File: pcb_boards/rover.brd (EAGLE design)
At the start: 2.5 x 2.5 mm, 16 parts, among them IC1 MC33269ST-5.0T3, J1 B02B-PASK(LF)(SN)

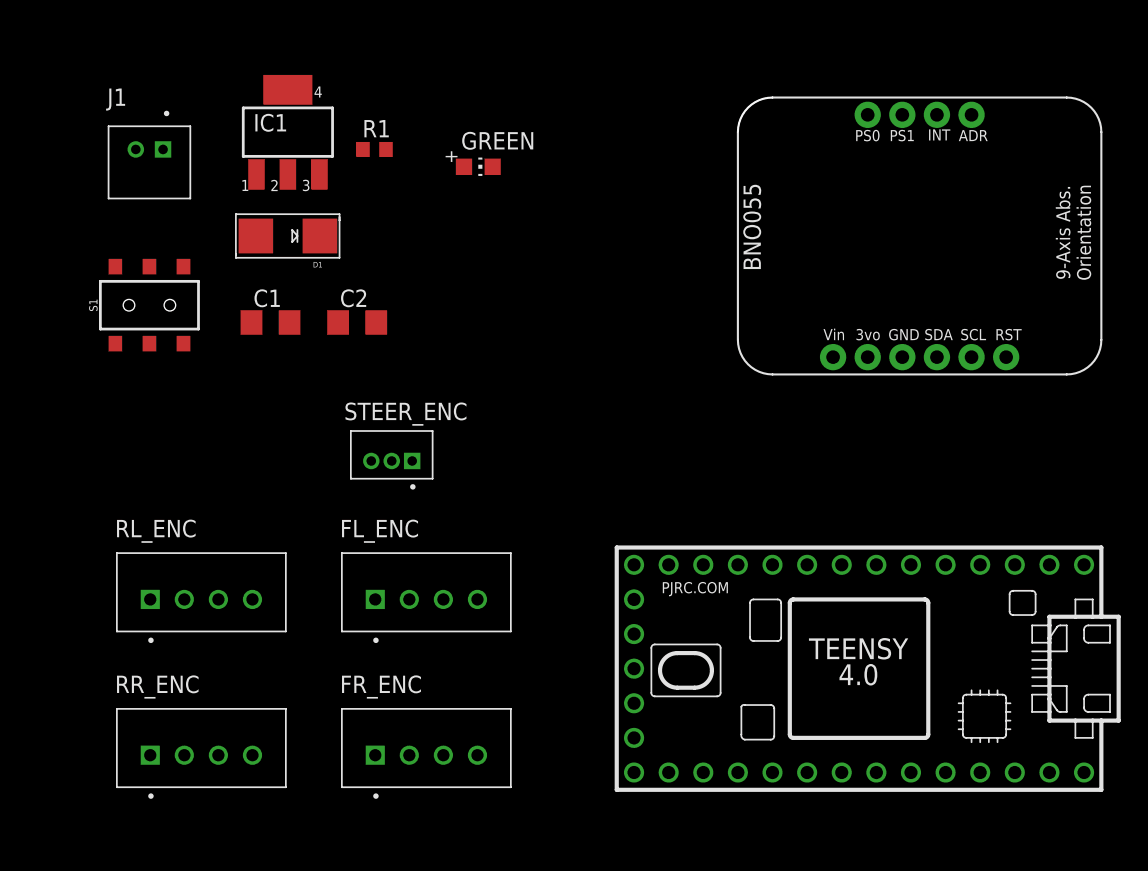
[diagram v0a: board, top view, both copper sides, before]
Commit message: finished pcb, added BOM
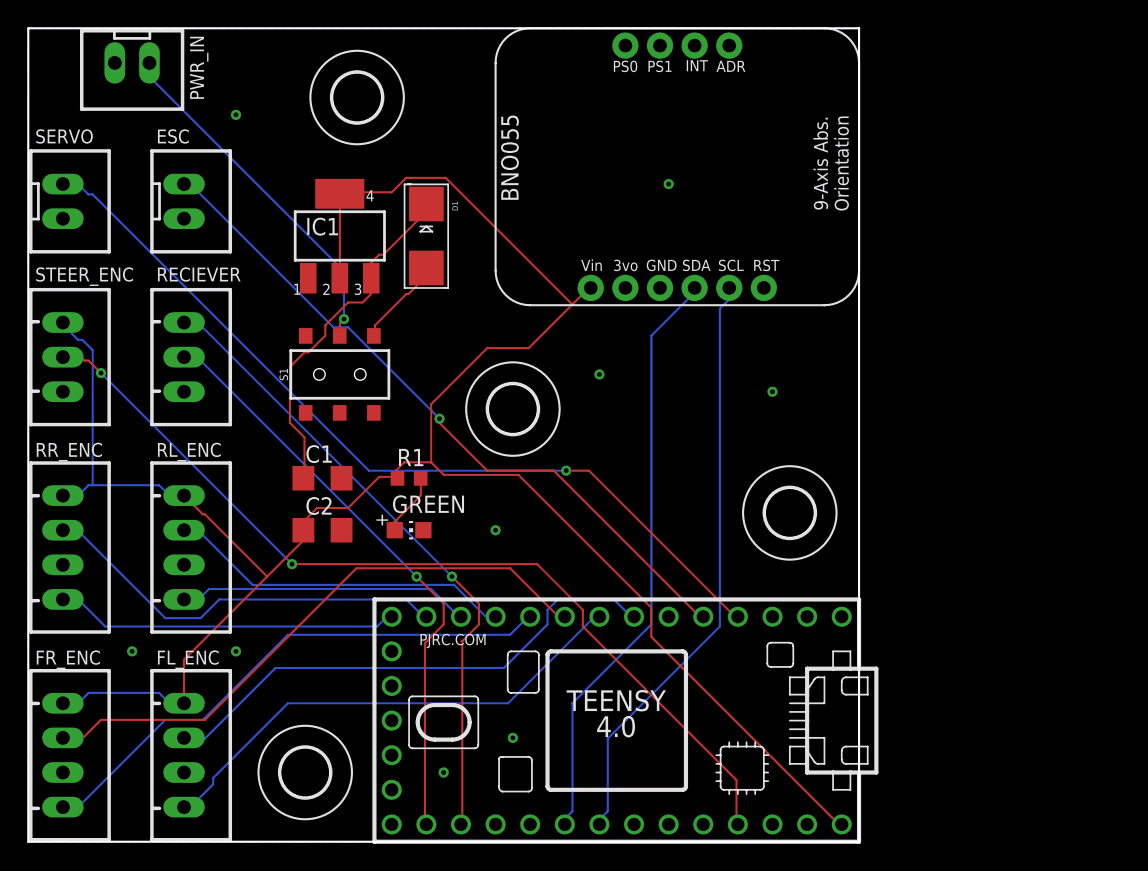
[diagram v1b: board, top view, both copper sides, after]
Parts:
- removed J1: B02B-PASK(LF)(SN), Headers:B02B-PASK(LF)(SN)
- added ESC, PWR_IN, SERVO: JST-XH-02-PIN-LONG-PAD, Rembrandt Electronics - JST XH Connectors v1-0:JST-XH-02-PACKAGE-LONG-PAD
- added RECIEVER: JST-XH-03-PIN-LONG-PAD, Rembrandt Electronics - JST XH Connectors v1-0:JST-XH-03-PACKAGE-LONG-PAD
- added U$4, U$6, U$7, U$8: (no value), holes:3,6
- FL_ENC, FR_ENC, RL_ENC, RR_ENC: value B4B-XH-A(LF)(SN) -> JST-XH-04-PIN-LONG-PAD; device Headers:B4B-XH-A(LF)(SN) -> Rembrandt Electronics - JST XH Connectors v1-0:JST-XH-04-PACKAGE-LONG-PAD
- STEER_ENC: value B3B-ZR(LF)(SN) -> JST-XH-03-PIN-LONG-PAD; device Headers:B3B-ZR(LF)(SN) -> Rembrandt Electronics - JST XH Connectors v1-0:JST-XH-03-PACKAGE-LONG-PAD
- moved GREEN 27.1 mm to (43.2, 16.5)
- moved FR_ENC 26.7 mm to (17.8, 0.00), turned to 270 degrees
- moved STEER_ENC 25.3 mm to (17.8, 29.2), turned to 270 degrees
- moved R1 24.3 mm to (43.2, 20.3)
- moved FL_ENC 21.1 mm to (26.7, 0.00), turned to 270 degrees
- moved JP3 18.5 mm to (62.9, 34.3)
- moved JP4 18.5 mm to (62.9, 52.1)
- moved RR_ENC 18.3 mm to (17.8, 15.2), turned to 270 degrees
- moved U$5 18.2 mm to (58.4, 2.54)
- moved C2 15.5 mm to (36.8, 16.5)
- moved S1 14.9 mm to (38.1, 27.9)
- moved C1 12.0 mm to (36.8, 20.3)
- moved D1 10.2 mm to (44.5, 38.1), turned to 270 degrees
- moved IC1 8.52 mm to (38.1, 38.1)
- moved RL_ENC 4.02 mm to (26.7, 15.2), turned to 270 degrees
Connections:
- net ESC: now also ESC.1
- net GND: now also ESC.2, PWR_IN.2, RECIEVER.3, SERVO.2; no longer J1.2
- net PWRIN: now also PWR_IN.1; no longer J1.1
- net REC_ESC: now also RECIEVER.1
- net REC_SERVO: now also RECIEVER.2
- net SERVO: now also SERVO.1
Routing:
- net +5V: track 0.00 -> 158.7 mm
- net STEER_ENC: track 0.00 -> 66.3 mm, vias 0 -> 2
- net SERVO: track 0.00 -> 62.7 mm, vias 0 -> 1
- net ESC: track 0.00 -> 51.5 mm, vias 0 -> 1
- net REC_ESC: track 0.00 -> 47.0 mm, vias 0 -> 1
- net FR_ENC_A: track 0.00 -> 43.5 mm
- net REC_SERVO: track 0.00 -> 43.4 mm, vias 0 -> 1
- net SDA_5V: track 0.00 -> 43.4 mm
- net SCL_5V: track 0.00 -> 43.4 mm
- net FR_ENC_B: track 0.00 -> 40.1 mm
- net FL_ENC_A: track 0.00 -> 38.4 mm
- net FL_ENC_B: track 0.00 -> 36.6 mm
- net RR_ENC_A: track 0.00 -> 30.4 mm
- net PWRIN: track 0.00 -> 26.1 mm, vias 0 -> 1
- net N$2: track 0.00 -> 25.7 mm
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- added copper zone on layer 1, net GND
- added copper zone on layer 16, net GND
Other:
- board size 2.5 x 2.5 mm -> 61 x 59.7 mm
